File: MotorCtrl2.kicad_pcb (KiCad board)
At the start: 2 copper layers, 47 x 52.1 mm, 12 parts, among them J1 Conn_01x02_Female, J2 Conn_01x02_Female, J3 Conn_01x02_Female, Q1 BS108, Q2 IRLB8721PBF

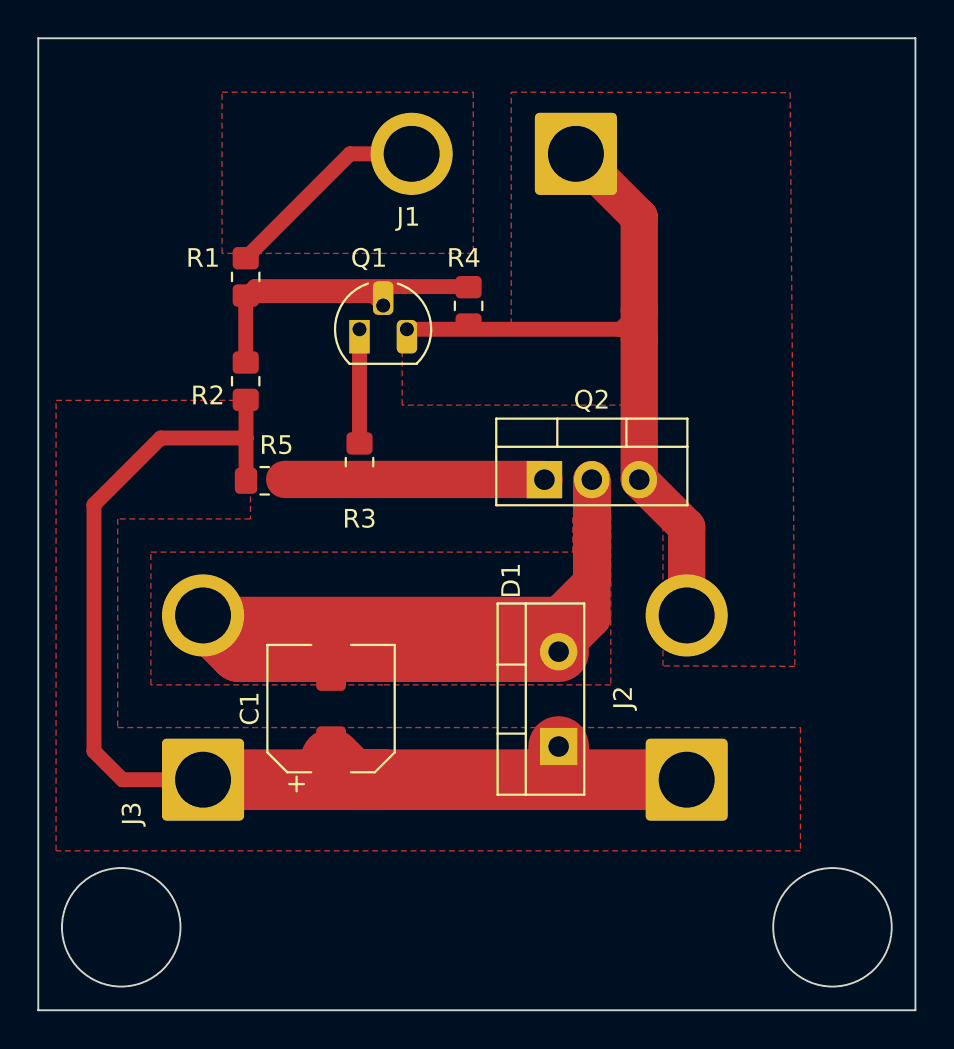
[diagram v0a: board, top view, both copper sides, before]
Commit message: ed
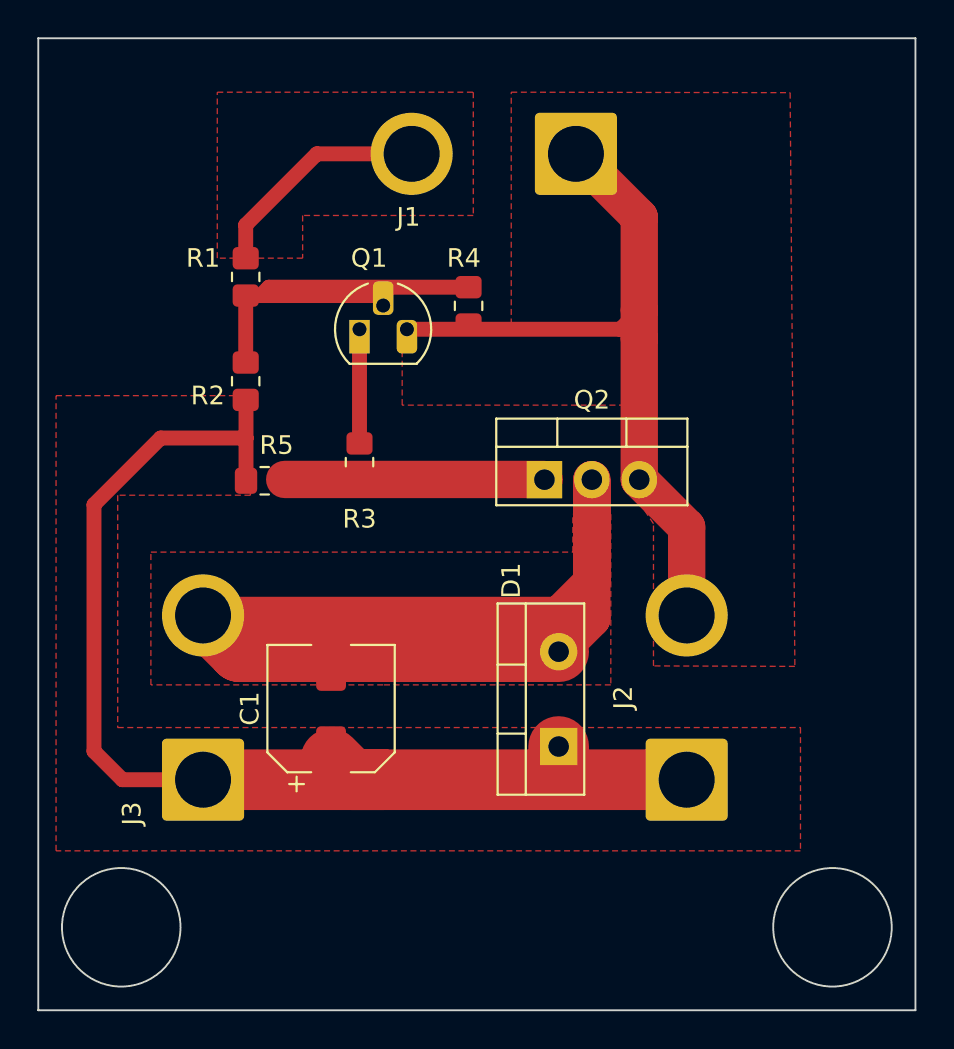
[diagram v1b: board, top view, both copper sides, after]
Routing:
- net Net-(Q1-Pad2): track 23.3 -> 21.8 mm
- net Net-(J1-Pad2): track 11.2 -> 12.3 mm
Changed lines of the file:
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@@
   (segment (start 34.036 244.348) (end 34.036 250.464) (width 0.8) (layer "F.Cu") (net 3))
   (segment (start 27.94 242.542) (end 27.94 246.13) (width 0.8) (layer "F.Cu") (net 4))
-  (segment (start 27.94 242.542) (end 28.42 242.062) (width 0.8) (layer "F.Cu") (net 4))
-  (segment (start 34.77 242.542) (end 35.306 243.078) (width 0.8) (layer "F.Cu") (net 4))
-  (segment (start 27.94 242.542) (end 34.77 242.542) (width 0.8) (layer "F.Cu") (net 4))
-  (segment (start 39.846 242.062) (end 39.878 242.094) (width 0.8) (layer "F.Cu") (net 4))
-  (segment (start 28.42 242.062) (end 39.846 242.062) (width 0.8) (layer "F.Cu") (net 4))
+  (segment (start 28.73 242.542) (end 34.77 242.542) (width 0.8) (layer "F.Cu") (net 4))
+  (segment (start 39.878 242.094) (end 29.178 242.094) (width 0.8) (layer "F.Cu") (net 4))
+  (segment (start 27.94 242.542) (end 28.73 242.542) (width 0.8) (layer "F.Cu") (net 4))
+  (segment (start 29.178 242.094) (end 28.73 242.542) (width 0.8) (layer "F.Cu") (net 4))
+  (segment (start 27.94 242.542) (end 27.968 242.57) (width 0.8) (layer "F.Cu") (net 4))
   (segment (start 48.006 244.348) (end 49.022 243.332) (width 0.8) (layer "F.Cu") (net 5))
   (segment (start 49.022 252.405) (end 49.022 244.856) (width 2) (layer "F.Cu") (net 5))
@@
   (segment (start 51.562 259.678) (end 51.562 254.945) (width 2) (layer "F.Cu") (net 5))
   (segment (start 51.562 254.945) (end 49.022 252.405) (width 2) (layer "F.Cu") (net 5))
-  (segment (start 33.528 234.95) (end 36.83 234.95) (width 0.8) (layer "F.Cu") (net 6))
-  (segment (start 27.94 240.538) (end 33.528 234.95) (width 0.8) (layer "F.Cu") (net 6))
-  (segment (start 27.94 240.542) (end 27.94 240.538) (width 0.8) (layer "F.Cu") (net 6))
+  (segment (start 27.94 240.542) (end 27.94 238.76) (width 0.8) (layer "F.Cu") (net 6))
+  (segment (start 27.94 238.76) (end 31.75 234.95) (width 0.8) (layer "F.Cu") (net 6))
+  (segment (start 31.75 234.95) (end 36.83 234.95) (width 0.8) (layer "F.Cu") (net 6))
   (segment (start 30.027 252.393) (end 43.93 252.393) (width 2) (layer "F.Cu") (net 7))
   (segment (start 43.93 252.393) (end 43.942 252.405) (width 0.8) (layer "F.Cu") (net 7))
@@
     (polygon
       (pts
-        (xy 40.132 240.284)
-        (xy 26.67 240.284)
-        (xy 26.67 231.648)
+        (xy 40.132 238.252)
+        (xy 30.988 238.252)
+        (xy 30.988 240.538)
+        (xy 26.416 240.538)
+        (xy 26.416 231.648)
         (xy 40.132 231.648)
       )
@@
       (pts
         (xy 57.358027 262.40757)
-        (xy 50.292 262.382)
-        (xy 50.292 254.762)
+        (xy 49.784 262.382)
+        (xy 49.784 254.762)
         (xy 48.26 252.476)
         (xy 48.26 248.412)
@@
     (connect_pads yes (clearance 0.5))
     (min_thickness 0.254) (filled_areas_thickness no)
-    (fill yes (thermal_gap 0.508) (thermal_bridge_width 0.508))
+    (fill (thermal_gap 0.508) (thermal_bridge_width 0.508))
     (polygon
       (pts
-        (xy 28.194 254.508)
-        (xy 21.082 254.508)
+        (xy 28.194 253.238)
+        (xy 21.082 253.238)
         (xy 21.082 265.684)
         (xy 57.658 265.684)
         (xy 57.658 272.288)
         (xy 17.78 272.288)
-        (xy 17.78 248.158)
-        (xy 28.194 248.158)
+        (xy 17.78 247.904)
+        (xy 28.194 247.904)
       )
     )
